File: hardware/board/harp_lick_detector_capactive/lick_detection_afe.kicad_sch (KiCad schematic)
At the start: 74 parts, among them J3 Conn_Triaxial, U10 ADA4891-2, U13 ADS7049, U14 MAX4564EKA, U6 ADA4891-4, U7 LTC6268xS8-10, U8 REF2025, U9 TS5A9411DCKR

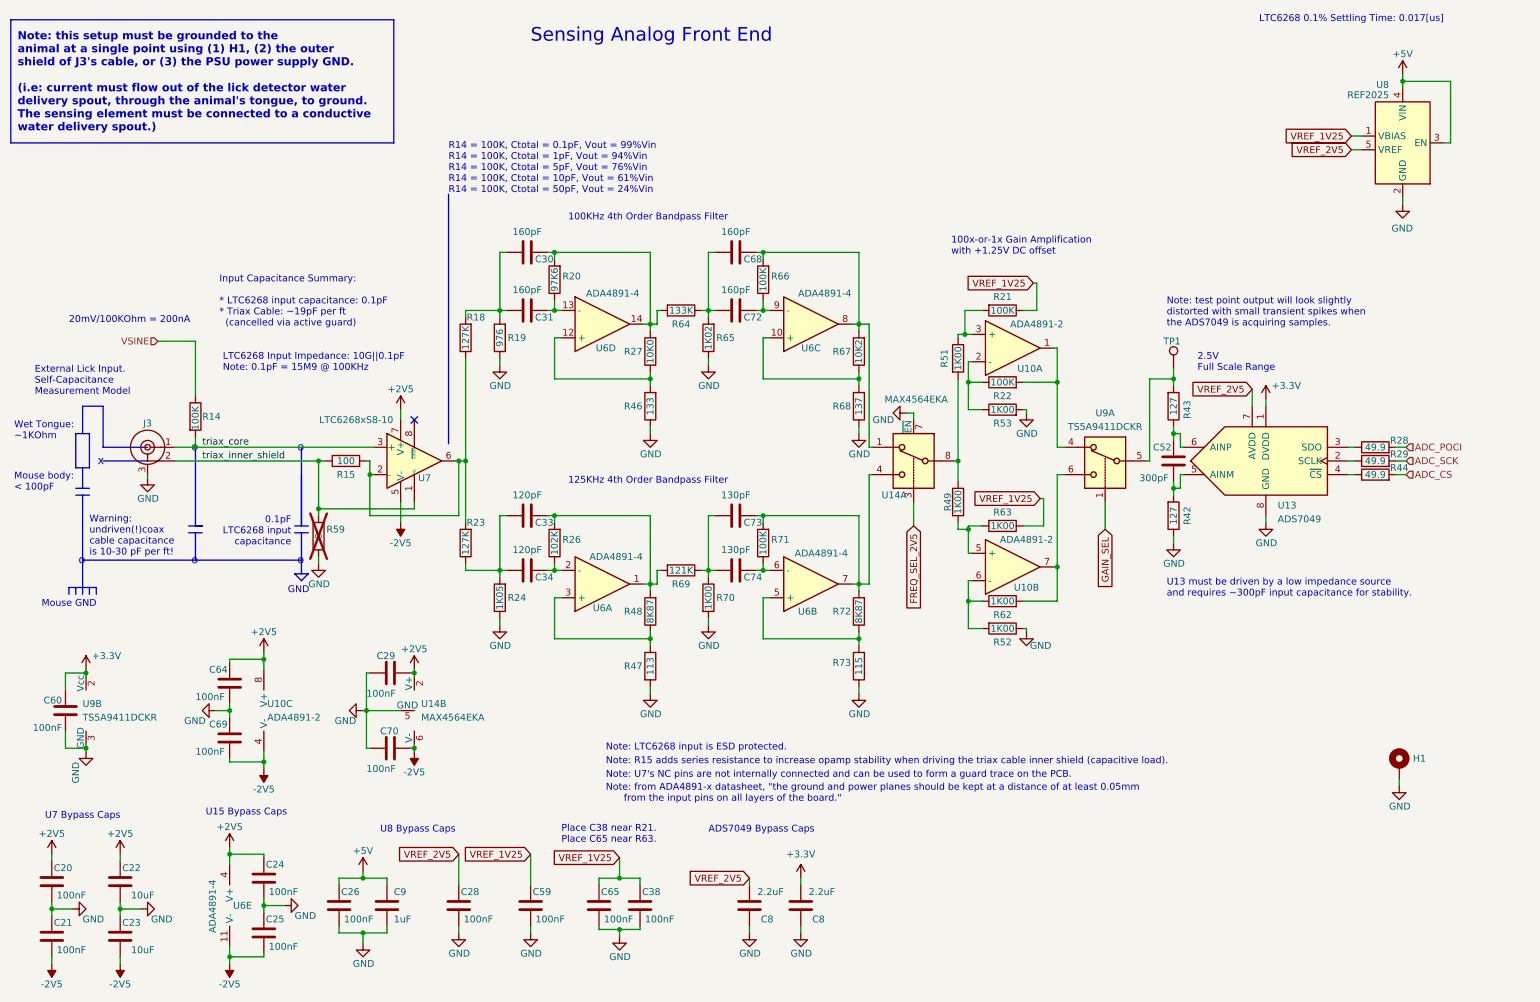
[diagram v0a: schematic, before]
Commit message: finish rev8
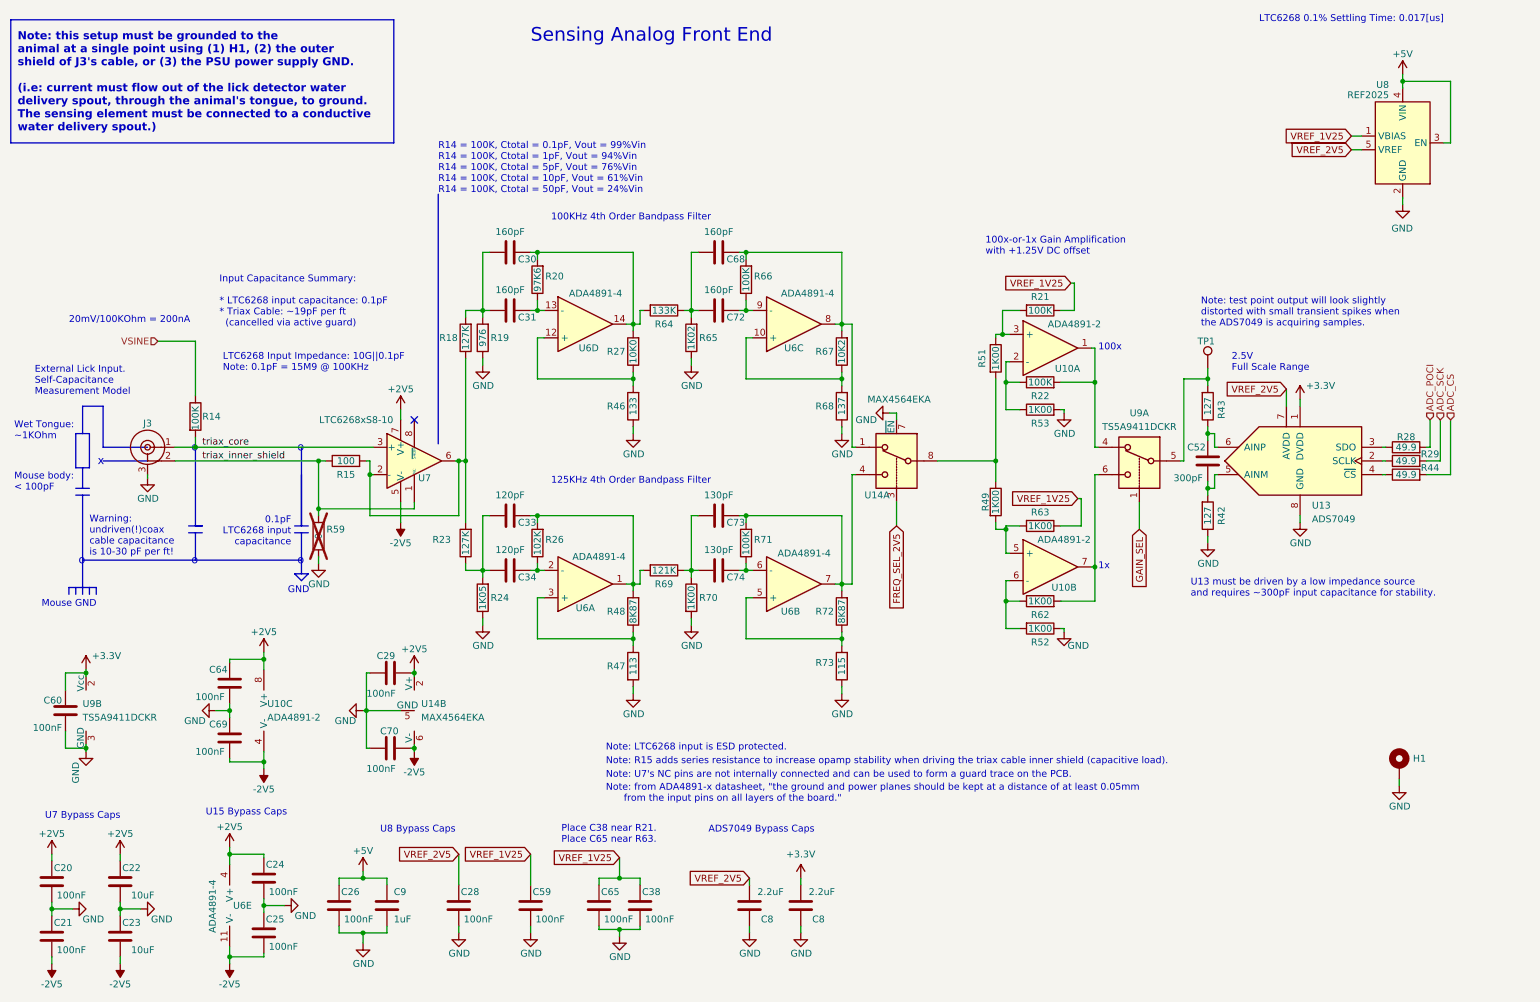
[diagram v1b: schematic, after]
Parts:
- R59: Alternate (none) -> n/a; Link (none) -> n/a; Manufacturer (none) -> n/a; Manufacturer Number (none) -> n/a
- TP1: Alternate (none) -> n/a; Link (none) -> n/a
- U14: Link (none) -> https://www.digikey.com/en/products/detail/analog-devices-i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; Manufacturer (none) -> Analog Devices Inc./Maxim Integrated; Manufacturer Number (none) -> MAX4564EKA+T
- U9: Link (none) -> https://www.digikey.com/en/products/detail/texas-instrument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; Manufacturer (none) -> Texas Instruments; Manufacturer Number (none) -> TS5A9411DCKR
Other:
- note added: "100x"
- note added: "1x"
- moved on the sheet: C30, C31, C33, C34, C52, C68, C72, C73, C74, R19, R20, R21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
